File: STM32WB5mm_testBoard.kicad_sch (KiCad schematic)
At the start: 24 parts, among them J1 FFMD-10-01, J2 ZW-40-XX-X-S-XXX-XXX, J3 ZW-40-XX-X-S-XXX-XXX, J4 MTMM-102-05-G-S-175, P1 0475890001, U1 STM32WB5MMG, U2 LD3985M33R_SOT23, U3 USBLC6-2P6

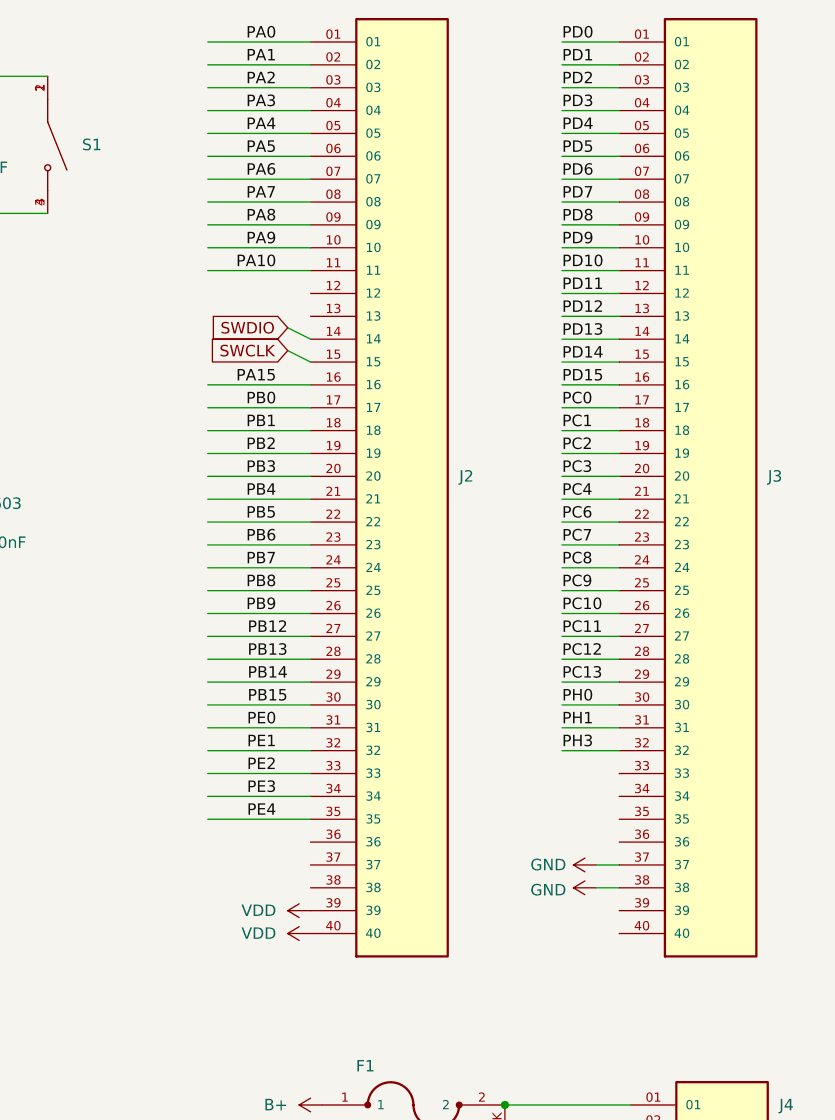
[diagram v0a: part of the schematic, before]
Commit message: 5
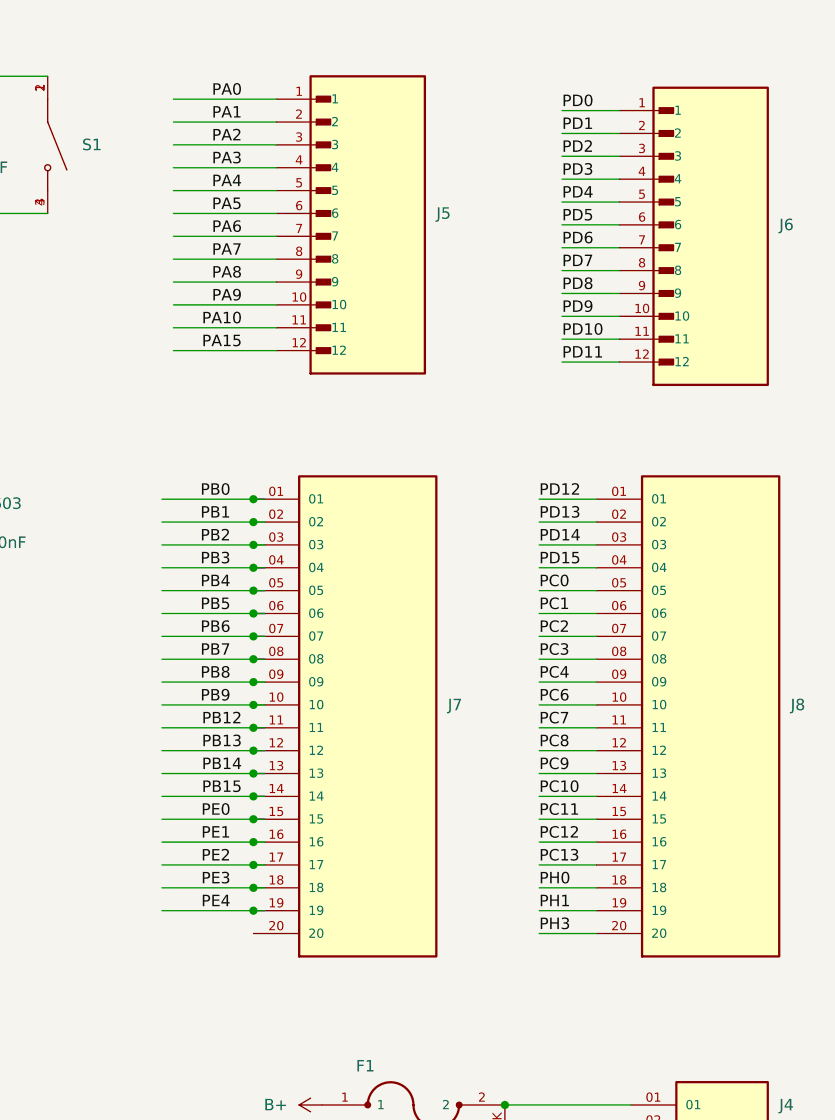
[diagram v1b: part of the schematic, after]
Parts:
- removed J2, J3: ZW-40-XX-X-S-XXX-XXX, ZW-40-XX-X-S-XXX-XXX:SAMTEC_ZW-40-XX-X-S-XXX-XXX, symbol ZW-40-XX-X-S-XXX-XXX:ZW-40-XX-X-S-XXX-XXX
- added J5, J6: M20-9991246, M20-9991246:HARWIN_M20-9991246, symbol M20-9991246:M20-9991246
- added J7, J8: ZW-20-09-L-S-250-320, ZW-20-09-L-S-250-320:SAMTEC_ZW-20-09-L-S-250-320, symbol ZW-20-09-L-S-250-320:ZW-20-09-L-S-250-320
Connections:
- net PA0: now also J5.1
- net PA1: now also J5.2
- net PA10: now also J5.11
- net PA15: now also J5.12
- net PA2: now also J5.3
- net PA3: now also J5.4
- net PA4: now also J5.5
- net PA5: now also J5.6
- net PA6: now also J5.7
- net PA7: now also J5.8
- net PA8: now also J5.9
- net PA9: now also J5.10
- net PB0: now also J7.01
- net PB1: now also J7.02
- net PB12: now also J7.11
- net PB13: now also J7.12
- net PB14: now also J7.13
- net PB15: now also J7.14
- net PB2: now also J7.03
- net PB3: now also J7.04
- net PB4: now also J7.05
- net PB5: now also J7.06
- net PB6: now also J7.07
- net PB7: now also J7.08
- net PB8: now also J7.09
- net PB9: now also J7.10
- net PC0: now also J8.05
- net PC1: now also J8.06
- net PC10: now also J8.14
- net PC11: now also J8.15
- net PC12: now also J8.16
- net PC13: now also J8.17
- net PC2: now also J8.07
- net PC3: now also J8.08
- net PC4: now also J8.09
- net PC6: now also J8.10
- net PC7: now also J8.11
- net PC8: now also J8.12
- net PC9: now also J8.13
- net PD0: now also J6.1
- net PD1: now also J6.2
- net PD10: now also J6.11
- net PD11: now also J6.12
- net PD12: now also J8.01
- net PD13: now also J8.02
- net PD14: now also J8.03
- net PD15: now also J8.04
- net PD2: now also J6.3
- net PD3: now also J6.4
- net PD4: now also J6.5
- net PD5: now also J6.6
- net PD6: now also J6.7
- net PD7: now also J6.8
- net PD8: now also J6.9
- net PD9: now also J6.10
- net PE0: now also J7.15
- net PE1: now also J7.16
- net PE2: now also J7.17
- net PE3: now also J7.18
- net PE4: now also J7.19
- net PH0: now also J8.18
- net PH1: now also J8.19
- net PH3: now also J8.20
